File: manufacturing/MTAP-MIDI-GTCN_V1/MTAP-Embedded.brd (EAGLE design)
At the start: 42.5 x 45.1 mm, 61 parts, among them IC1 ESP32-WROOM-32UE-N8, IC2 AMS1117-3.3, IC3 TPS60402DBVT, J1 629105150521, X2 22-23-2021

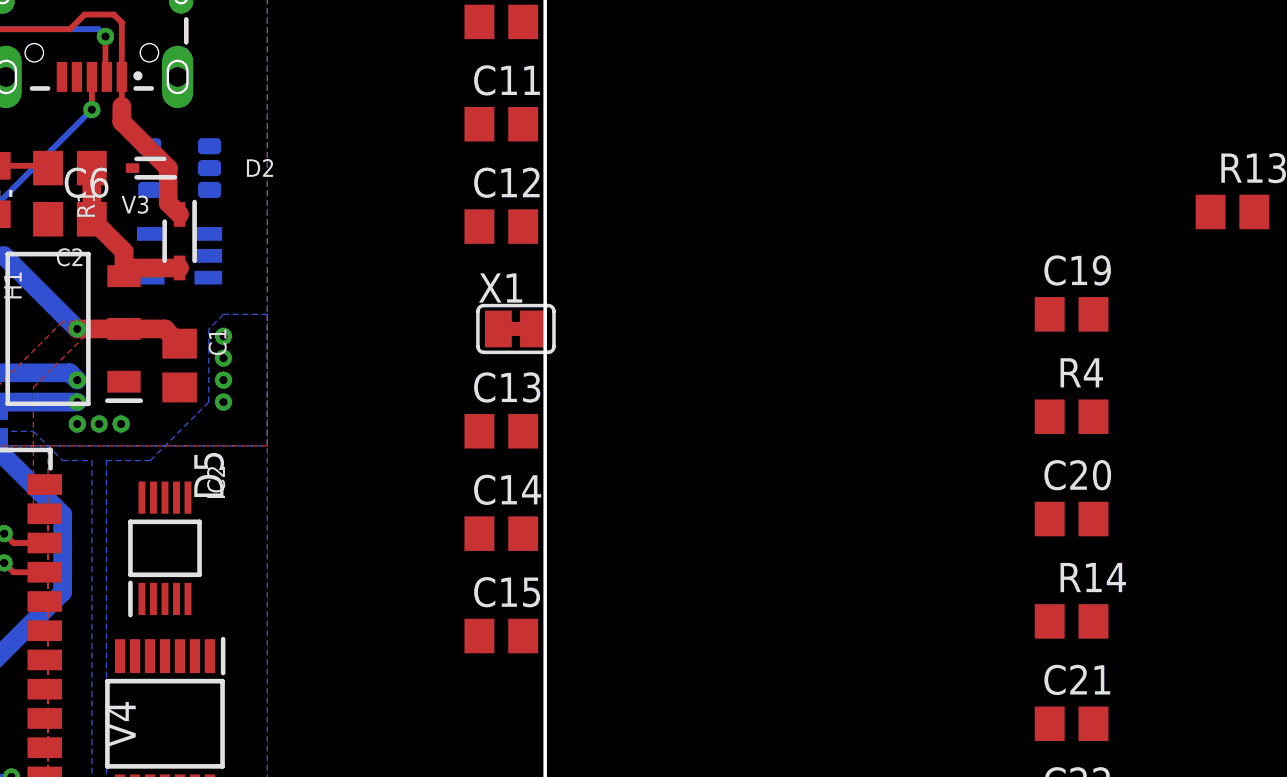
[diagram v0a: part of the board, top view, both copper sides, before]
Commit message: upd analog
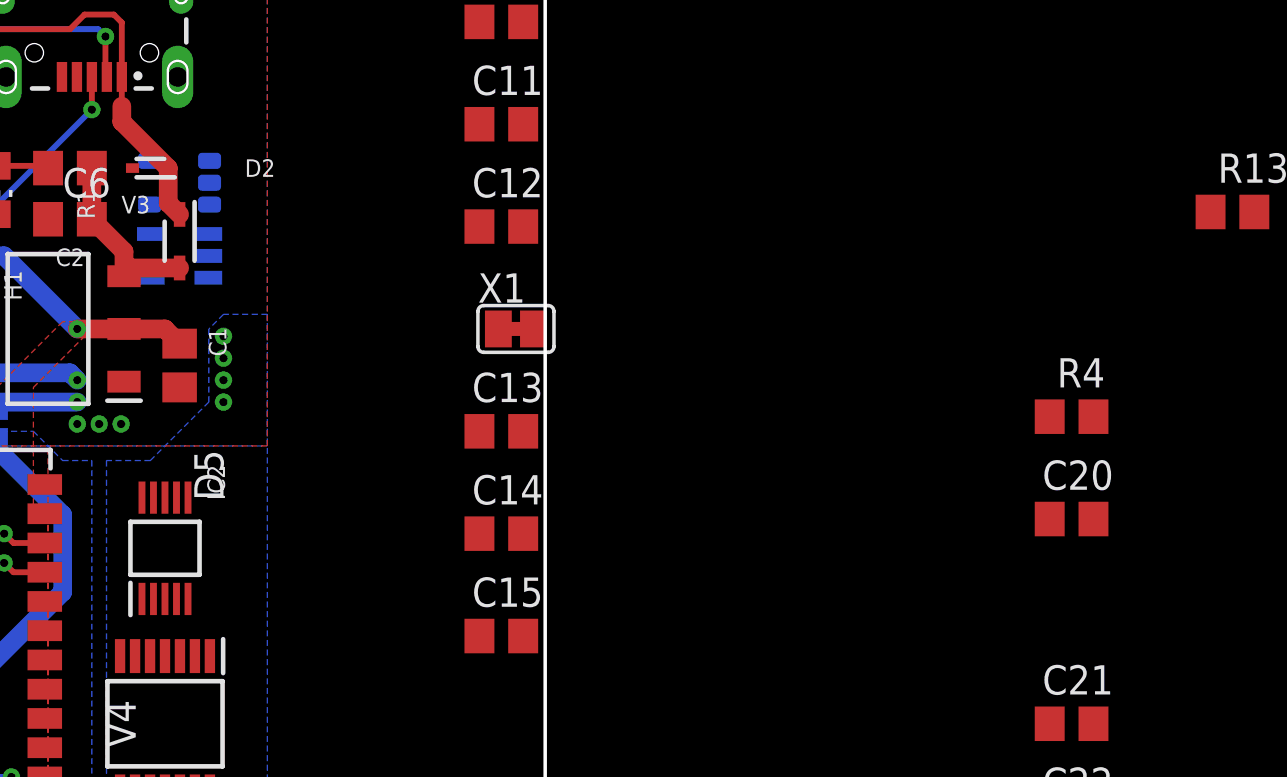
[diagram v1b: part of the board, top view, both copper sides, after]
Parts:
- removed C19: (no value), rcl_GruS:C0805
- removed R14: (no value), rcl_GruS:R0805
- C16: value (none) -> 10n
- C17: value (none) -> 180n
- C18: value (none) -> 10nF
- C20, C22: value (none) -> 100n
- C21, C23: value (none) -> 1u
- R12: value (none) -> 560R
- R13: value (none) -> 1k
- R3: value (none) -> 6k2
- moved N1 0.63 mm to (21.6, 49.5)
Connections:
- removed net N$13: C17.1, V4.6, V4.7
- net AINP: now also C17.1, V4.6, V4.7
